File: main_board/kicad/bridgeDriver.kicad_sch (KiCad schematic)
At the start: 1 part, among them U3 IR2133

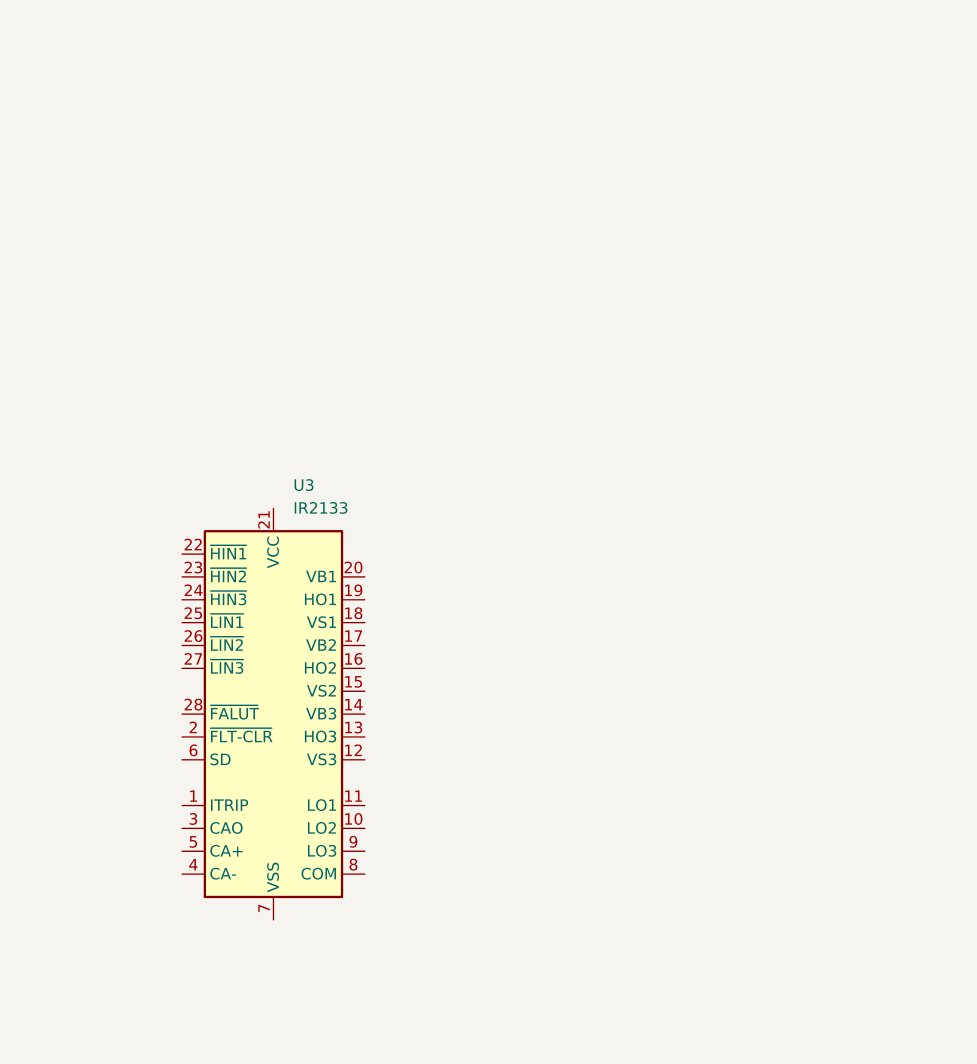
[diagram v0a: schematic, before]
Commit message: bridge driver almost done
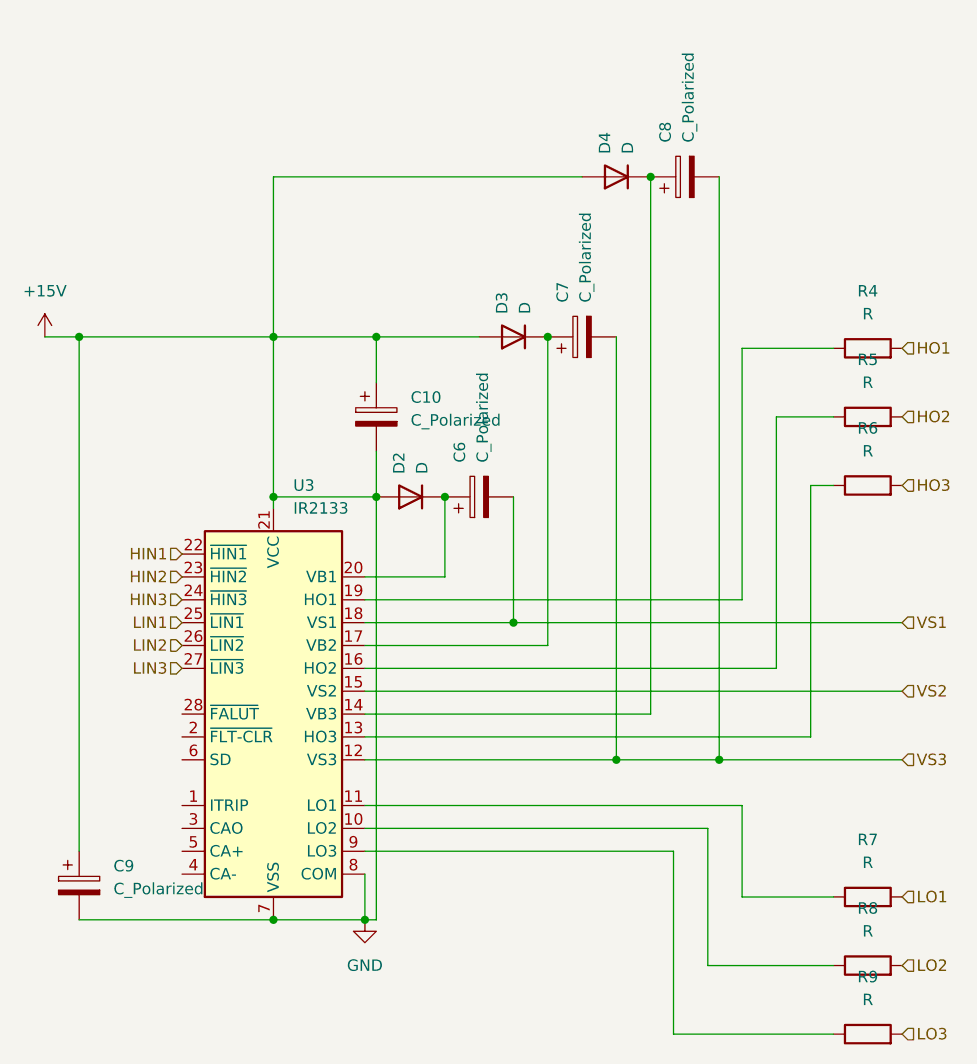
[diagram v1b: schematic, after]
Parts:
- added C10, C6, C7, C8, C9: C_Polarized, symbol Device:C_Polarized
- added D2, D3, D4: D, symbol Device:D
- added R4, R5, R6, R7, R8, R9: R, symbol Device:R
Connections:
- net at U3.10 (LO2): now also R8.1
- net at U3.11 (LO1): now also R7.1
- net VS3: now reaches U3.12 (VS3)
- net VS3: now also C7.2, C8.2
- net at U3.13 (HO3): now also R6.1
- net at U3.14 (VB3): now also C8.1, D4.1 (K)
- net VS2: now reaches U3.15 (VS2)
- net at U3.16 (HO2): now also R5.1
- net at U3.17 (VB2): now also C7.1, D3.1 (K)
- net VS1: now reaches U3.18 (VS1)
- net VS1: now also C6.2
- net at U3.19 (HO1): now also R4.1
- net at U3.20 (VB1): now also C6.1, D2.1 (K)
- net +15V: now reaches U3.21 (VCC)
- net +15V: now also U3.7 (VSS), U3.8 (COM), C10.1, C10.2, C9.1, C9.2, D2.2 (A), D3.2 (A), D4.2 (A)
- net HIN1: now reaches U3.22 (~{HIN1})
- net HIN2: now reaches U3.23 (~{HIN2})
- net HIN3: now reaches U3.24 (~{HIN3})
- net LIN1: now reaches U3.25 (~{LIN1})
- net LIN2: now reaches U3.26 (~{LIN2})
- net LIN3: now reaches U3.27 (~{LIN3})
- net at U3.9 (LO3): now also R9.1
- new net HO1: R4.2
- new net HO2: R5.2
- new net HO3: R6.2
- new net LO1: R7.2
- new net LO2: R8.2
- new net LO3: R9.2
